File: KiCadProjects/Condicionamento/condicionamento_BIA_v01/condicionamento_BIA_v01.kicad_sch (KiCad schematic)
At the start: 26 parts, among them J1 Vref, J2 tensoes, J3 sinais analogicos, J4 comunicacao / sinais digitais, J5 sinais_condicionados, J6 alimetacao_Master, U1 AD828AN, U2 BluePill_STM32F103C, U3 BluePill_STM32F103C

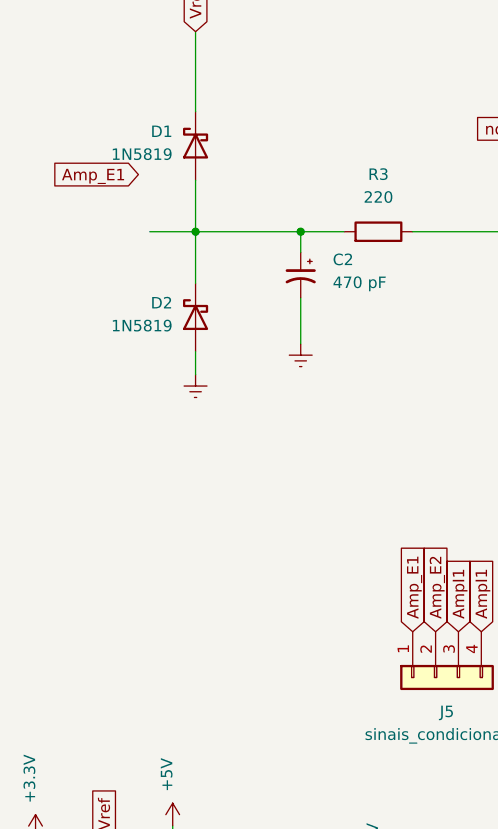
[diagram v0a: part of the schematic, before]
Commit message: PCB
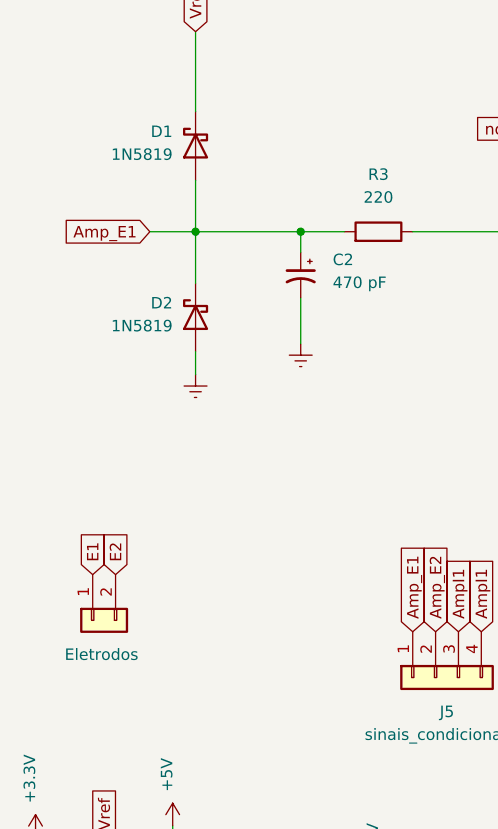
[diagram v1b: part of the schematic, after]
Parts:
- added J7: Eletrodos, Connector_PinHeader_2.54mm:PinHeader_1x02_P2.54mm_Horizontal, symbol Connector_Generic:Conn_01x02
- U1: footprint footprints:N_8_ADI -> AD828:N_8_ADI
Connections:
- net Amp_E1: now also C2.1, D1.2 (A), D2.1 (K), R3.2
- net E1: now also J7.1 (Pin_1)
- net E2: now also J7.2 (Pin_2)
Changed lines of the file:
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@@
     )
   )
-  (global_label "Amp_E1" (shape input) (at 34.29 106.68 180) (fields_autoplaced)
+  (global_label "Amp_E1" (shape input) (at 35.56 113.03 180) (fields_autoplaced)
     (effects (font (size 1.27 1.27)) (justify right))
-    (property "Intersheetrefs" "${INTERSHEET_REFS}" (at 24.1272 106.68 0)
+    (property "Intersheetrefs" "${INTERSHEET_REFS}" (at 25.3972 113.03 0)
       (effects (font (size 1.27 1.27)) (justify right) hide)
     )
@@
     )
   )
+  (global_label "E2" (shape input) (at 31.75 151.13 90) (fields_autoplaced)
+    (effects (font (size 1.27 1.27)) (justify left))
+    (property "Intersheetrefs" "${INTERSHEET_REFS}" (at 31.75 145.8657 90)
+      (effects (font (size 1.27 1.27)) (justify right) hide)
+    )
+  )
   (global_label "Amp_E1" (shape input) (at 64.77 157.48 90) (fields_autoplaced)
     (effects (font (size 1.27 1.27)) (justify left))
@@
     (property "Intersheetrefs" "${INTERSHEET_REFS}" (at 222.3927 105.41 0)
       (effects (font (size 1.27 1.27)) (justify left) hide)
+    )
+  )
+  (global_label "E1" (shape input) (at 29.21 151.13 90) (fields_autoplaced)
+    (effects (font (size 1.27 1.27)) (justify left))
+    (property "Intersheetrefs" "${INTERSHEET_REFS}" (at 29.21 145.8657 90)
+      (effects (font (size 1.27 1.27)) (justify right) hide)
     )
   )
@@
       (effects (font (size 1.524 1.524)))
     )
-    (property "Footprint" "footprints:N_8_ADI" (at 129.54 111.76 0)
+    (property "Footprint" "AD828:N_8_ADI" (at 129.54 111.76 0)
       (effects (font (size 1.27 1.27) italic) hide)
     )
@@
         )
       )
+    )
+  )
+  (symbol (lib_id "Connector_Generic:Conn_01x02") (at 29.21 156.21 90) (mirror x) (unit 1)
+    (in_bom yes) (on_board yes) (dnp no)
+    (property "Reference" "J7" (at 26.67 154.94 90)
+      (effects (font (size 1.27 1.27)) (justify left) hide)
+    )
+    (property "Value" "Eletrodos" (at 34.29 160.02 90)
+      (effects (font (size 1.27 1.27)) (justify left))
+    )
+    (property "Footprint" "Connector_PinHeader_2.54mm:PinHeader_1x02_P2.54mm_Horizontal" (at 29.21 156.21 0)
+      (effects (font (size 1.27 1.27)) hide)
+    )
+    (property "Datasheet" "~" (at 29.21 156.21 0)
+      (effects (font (size 1.27 1.27)) hide)
+    )
+    (pin "1")
+    (pin "2")
+    (instances
+      (project "condicionamento_BIA_v01"
+        (path "/f0ff92cf-26e5-4ab9-977d-5f9689e8a5d0"
+          (reference "J7") (unit 1)
+        )
+      )

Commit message: PCB
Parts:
- Brd1: footprint SSD1306:128x64OLED -> OLED_i2c:128x64OLED
- U2, U3: footprint BluePill_breakouts:BluePill_STM32F103C -> STM32_Bluepill:BluePill_STM32F103C
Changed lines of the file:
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@@
       (effects (font (size 1.27 1.27)) (justify right))
     )
-    (property "Footprint" "BluePill_breakouts:BluePill_STM32F103C" (at 128.27 48.26 0)
+    (property "Footprint" "STM32_Bluepill:BluePill_STM32F103C" (at 128.27 48.26 0)
       (effects (font (size 1.27 1.27)) hide)
     )
@@
       (effects (font (size 1.27 1.27)) (justify left))
     )
-    (property "Footprint" "SSD1306:128x64OLED" (at 153.67 67.31 0)
+    (property "Footprint" "OLED_i2c:128x64OLED" (at 153.67 67.31 0)
       (effects (font (size 1.27 1.27)) hide)
     )
@@
       (effects (font (size 1.27 1.27)) (justify right))
     )
-    (property "Footprint" "BluePill_breakouts:BluePill_STM32F103C" (at 256.54 46.99 0)
-      (effects (font (size 1.27 1.27)) hide)
-    )
+    (property "Footprint" "STM32_Bluepill:BluePill_STM32F103C" (at 256.54 46.99 0)
+      (effects (font (size 1.27 1.27)) hide)
+    )
